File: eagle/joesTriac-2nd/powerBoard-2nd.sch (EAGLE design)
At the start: 31 parts, among them IC1 7809, IC2 7805, IC3 7909, IC5 7805, J1 XF2E-0815-1, J2 XF2E-0815-1

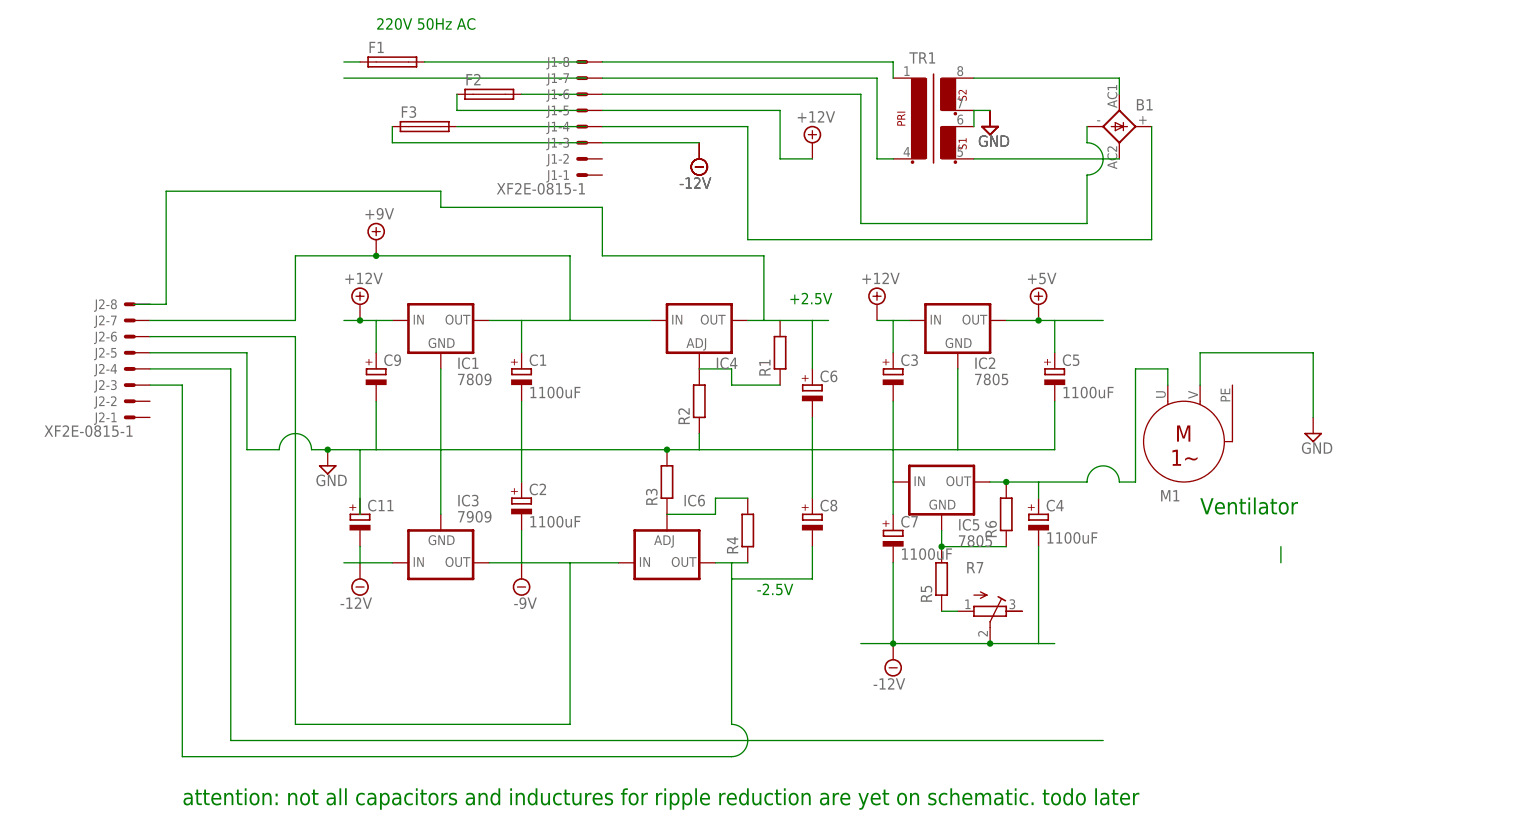
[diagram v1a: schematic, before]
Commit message: reg save-tested ok
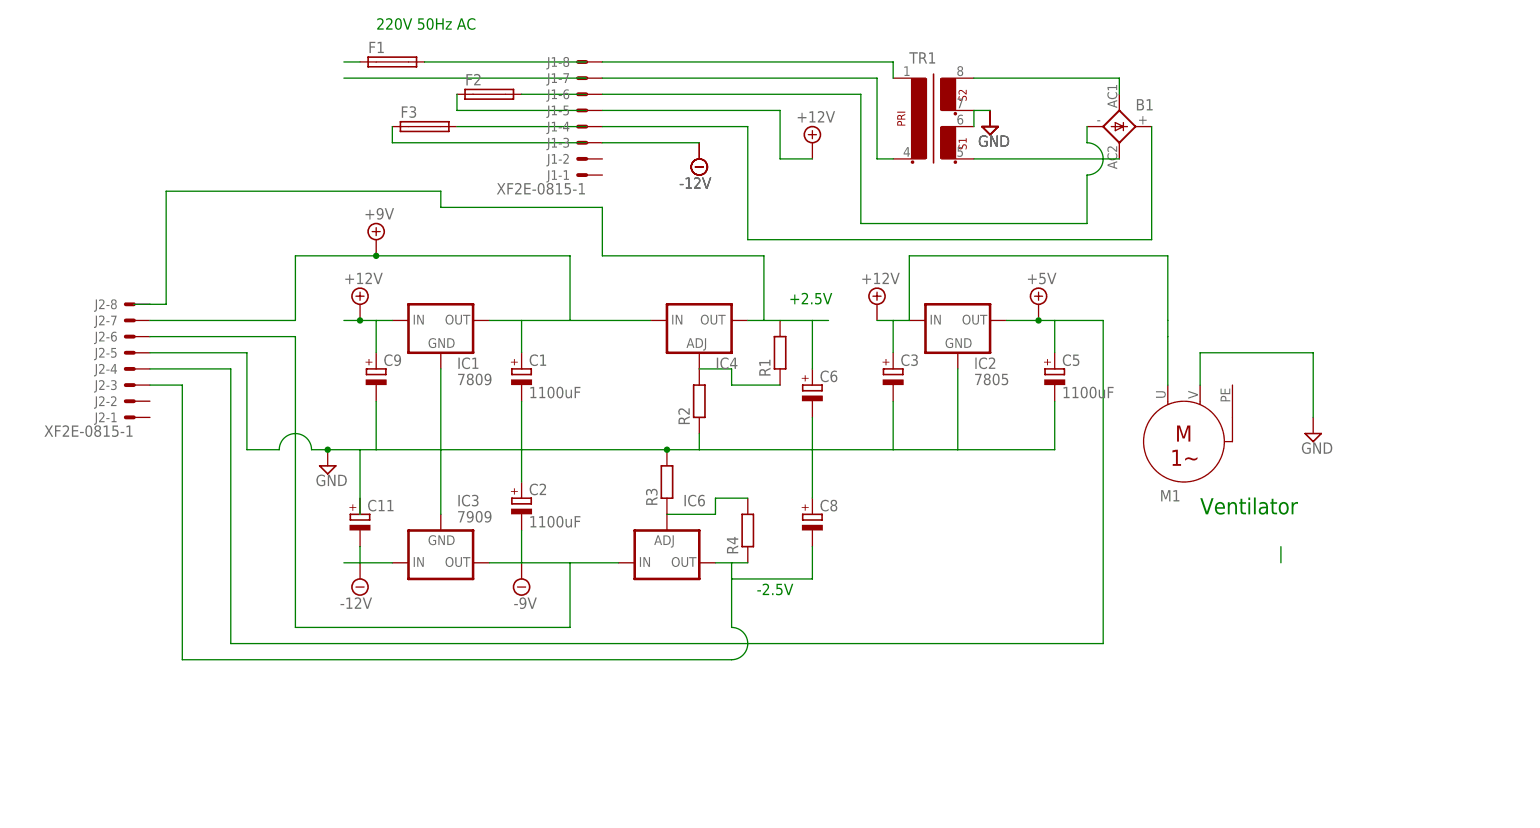
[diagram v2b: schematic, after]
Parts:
- removed C4, C7: 1100uF, resistor:CPOL-EUE22-6AXIAL
- removed IC5: 7805, v-reg:78LXX
- removed R5, R6: (no value), resistor:R-EU_0309/V
- removed R7: (no value), resistor:R-TRIMM3103
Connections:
- removed net N$10: J2-4.MS
- removed net N$16: C4.+, IC5.OUT, M1.U, R6.2
- removed net N$17: R5.1, R7.A
- removed net N$20: IC5.GND, R5.2, R6.1
- net +12V: now also M1.U
- net +5V: now also J2-4.MS
- net -12V: no longer C4.-, C7.-, R7.S
- net GND: no longer C7.+, IC5.IN
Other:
- note removed: "attention: not all capacitors and inductures for ripple reduction are yet on schematic. todo later"
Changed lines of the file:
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@@
 <layer number="97" name="Info" color="7" fill="1" visible="yes" active="yes"/>
 <layer number="98" name="Guide" color="6" fill="1" visible="yes" active="yes"/>
-<layer number="99" name="SpiceOrder" color="5" fill="1" visible="yes" active="yes"/>
 </layers>
 <schematic xreflabel="%F%N/%S.%C%R" xrefpart="/%S.%C%R">
@@
 <part name="SUPPLY13" library="supply2" deviceset="+5V" device=""/>
 <part name="C5" library="resistor" deviceset="CPOL-EU" device="E22-6AXIAL" value="1100uF"/>
-<part name="IC5" library="v-reg" deviceset="78LXX" device="" value="7805"/>
-<part name="SUPPLY14" library="supply2" deviceset="-12V" device=""/>
-<part name="C4" library="resistor" deviceset="CPOL-EU" device="E22-6AXIAL" value="1100uF"/>
-<part name="C7" library="resistor" deviceset="CPOL-EU" device="E22-6AXIAL" value="1100uF"/>
-<part name="R5" library="resistor" deviceset="R-EU_" device="0309/V"/>
-<part name="R7" library="resistor" deviceset="R-TRIMM" device="3103"/>
-<part name="R6" library="resistor" deviceset="R-EU_" device="0309/V"/>
 </parts>
 <sheets>
@@
 <text x="76.2" y="-38.1" size="2.54" layer="91">Ventilator</text>
 <text x="5.08" y="-50.8" size="1.778" layer="91">  -2.5V</text>
-<text x="-83.82" y="-83.82" size="2.54" layer="91">attention: not all capacitors and inductures for ripple reduction are yet on schematic. todo later</text>
 </plain>
 <instances>
@@
 <instance part="SUPPLY13" gate="+5V" x="50.8" y="-5.08"/>
 <instance part="C5" gate="G$1" x="53.34" y="-15.24"/>
-<instance part="IC5" gate="1" x="35.56" y="-33.02"/>
-<instance part="SUPPLY14" gate="G$1" x="27.94" y="-60.96"/>
-<instance part="C4" gate="G$1" x="50.8" y="-38.1"/>
-<instance part="C7" gate="G$1" x="27.94" y="-40.64"/>
-<instance part="R5" gate="G$1" x="35.56" y="-48.26" rot="R90"/>
-<instance part="R7" gate="G$1" x="43.18" y="-53.34" rot="R270"/>
-<instance part="R6" gate="G$1" x="45.72" y="-38.1" rot="R90"/>
 </instances>
 <busses>
@@
 <pinref part="C5" gate="G$1" pin="-"/>
 <wire x1="53.34" y1="-27.94" x2="53.34" y2="-20.32" width="0.1524" layer="91"/>
-<wire x1="27.94" y1="-27.94" x2="27.94" y2="-33.02" width="0.1524" layer="91"/>
-<pinref part="IC5" gate="1" pin="IN"/>
-<pinref part="C7" gate="G$1" pin="+"/>
-<wire x1="27.94" y1="-33.02" x2="27.94" y2="-38.1" width="0.1524" layer="91"/>
 </segment>
 </net>
@@
 </segment>
 <segment>
-<pinref part="SUPPLY9" gate="+12V" pin="+12V"/>
 <pinref part="IC2" gate="1" pin="IN"/>
 <wire x1="30.48" y1="-7.62" x2="27.94" y2="-7.62" width="0.1524" layer="91"/>
+<pinref part="SUPPLY9" gate="+12V" pin="+12V"/>
+<pinref part="C3" gate="G$1" pin="+"/>
 <wire x1="27.94" y1="-7.62" x2="25.4" y2="-7.62" width="0.1524" layer="91"/>
-<pinref part="C3" gate="G$1" pin="+"/>
 <wire x1="27.94" y1="-12.7" x2="27.94" y2="-7.62" width="0.1524" layer="91"/>
+<wire x1="30.48" y1="-7.62" x2="30.48" y2="2.54" width="0.1524" layer="91"/>
+<wire x1="30.48" y1="2.54" x2="71.12" y2="2.54" width="0.1524" layer="91"/>
+<pinref part="M1" gate="1" pin="U"/>
+<wire x1="71.12" y1="-7.62" x2="71.12" y2="-10.16" width="0.1524" layer="91"/>
+<wire x1="71.12" y1="-10.16" x2="71.12" y2="-17.78" width="0.1524" layer="91"/>
+<wire x1="71.12" y1="2.54" x2="71.12" y2="-7.62" width="0.1524" layer="91"/>
 </segment>
 </net>
@@
 <pinref part="C11" gate="G$1" pin="-"/>
 <wire x1="-55.88" y1="-43.18" x2="-55.88" y2="-45.72" width="0.1524" layer="91"/>
-</segment>
-<segment>
-<wire x1="22.86" y1="-58.42" x2="27.94" y2="-58.42" width="0.1524" layer="91"/>
-<pinref part="SUPPLY14" gate="G$1" pin="-12V"/>
-<junction x="27.94" y="-58.42"/>
-<pinref part="C7" gate="G$1" pin="-"/>
-<wire x1="27.94" y1="-45.72" x2="27.94" y2="-58.42" width="0.1524" layer="91"/>
-<wire x1="50.8" y1="-58.42" x2="53.34" y2="-58.42" width="0.1524" layer="91"/>
-<pinref part="C4" gate="G$1" pin="-"/>
-<wire x1="50.8" y1="-43.18" x2="50.8" y2="-58.42" width="0.1524" layer="91"/>
-<wire x1="27.94" y1="-58.42" x2="43.18" y2="-58.42" width="0.1524" layer="91"/>
-<pinref part="R7" gate="G$1" pin="S"/>
-<wire x1="43.18" y1="-58.42" x2="50.8" y2="-58.42" width="0.1524" layer="91"/>
-<junction x="43.18" y="-58.42"/>
 </segment>
 </net>
@@
 <wire x1="-35.56" y1="-45.72" x2="-30.48" y2="-45.72" width="0.1524" layer="91"/>
 <wire x1="-22.86" y1="-45.72" x2="-30.48" y2="-45.72" width="0.1524" layer="91"/>
-<wire x1="-22.86" y1="-45.72" x2="-22.86" y2="-71.12" width="0.1524" layer="91"/>
-<wire x1="-22.86" y1="-71.12" x2="-66.04" y2="-71.12" width="0.1524" layer="91"/>
-<wire x1="-66.04" y1="-71.12" x2="-66.04" y2="-10.16" width="0.1524" layer="91"/>
+<wire x1="-22.86" y1="-45.72" x2="-22.86" y2="-55.88" width="0.1524" layer="91"/>
+<wire x1="-22.86" y1="-55.88" x2="-66.04" y2="-55.88" width="0.1524" layer="91"/>
+<wire x1="-66.04" y1="-55.88" x2="-66.04" y2="-10.16" width="0.1524" layer="91"/>
 <pinref part="IC6" gate="1" pin="IN"/>
 <wire x1="-22.86" y1="-45.72" x2="-15.24" y2="-45.72" width="0.1524" layer="91"/>
@@
 <wire x1="0" y1="-45.72" x2="2.54" y2="-45.72" width="0.1524" layer="91"/>
 <wire x1="2.54" y1="-45.72" x2="2.54" y2="-48.26" width="0.1524" layer="91"/>
-<wire x1="2.54" y1="-48.26" x2="2.54" y2="-71.12" width="0.1524" layer="91"/>
-<wire x1="2.54" y1="-71.12" x2="2.54" y2="-76.2" width="0.1524" layer="91" curve="-180"/>
-<wire x1="2.54" y1="-76.2" x2="-83.82" y2="-76.2" width="0.1524" layer="91"/>
-<wire x1="-83.82" y1="-76.2" x2="-83.82" y2="-17.78" width="0.1524" layer="91"/>
+<wire x1="2.54" y1="-48.26" x2="2.54" y2="-55.88" width="0.1524" layer="91"/>
+<wire x1="2.54" y1="-55.88" x2="2.54" y2="-60.96" width="0.1524" layer="91" curve="-180"/>
+<wire x1="2.54" y1="-60.96" x2="-83.82" y2="-60.96" width="0.1524" layer="91"/>
+<wire x1="-83.82" y1="-60.96" x2="-83.82" y2="-17.78" width="0.1524" layer="91"/>
 <pinref part="J2" gate="-3" pin="MS"/>
 <wire x1="-83.82" y1="-17.78" x2="-88.9" y2="-17.78" width="0.1524" layer="91"/>
@@
 <net name="+5V" class="0">
 <segment>
+<pinref part="IC2" gate="1" pin="OUT"/>
+<wire x1="45.72" y1="-7.62" x2="50.8" y2="-7.62" width="0.1524" layer="91"/>
+<wire x1="50.8" y1="-7.62" x2="53.34" y2="-7.62" width="0.1524" layer="91"/>
 <wire x1="53.34" y1="-7.62" x2="60.96" y2="-7.62" width="0.1524" layer="91"/>
+<wire x1="60.96" y1="-7.62" x2="60.96" y2="-58.42" width="0.1524" layer="91"/>
+<wire x1="60.96" y1="-58.42" x2="-76.2" y2="-58.42" width="0.1524" layer="91"/>
+<wire x1="-76.2" y1="-58.42" x2="-76.2" y2="-15.24" width="0.1524" layer="91"/>
+<pinref part="J2" gate="-4" pin="MS"/>
+<wire x1="-76.2" y1="-15.24" x2="-88.9" y2="-15.24" width="0.1524" layer="91"/>
+<pinref part="SUPPLY13" gate="+5V" pin="+5V"/>
+<junction x="50.8" y="-7.62"/>
 <pinref part="C5" gate="G$1" pin="+"/>
 <wire x1="53.34" y1="-12.7" x2="53.34" y2="-7.62" width="0.1524" layer="91"/>
-<wire x1="50.8" y1="-7.62" x2="53.34" y2="-7.62" width="0.1524" layer="91"/>
-<pinref part="SUPPLY13" gate="+5V" pin="+5V"/>
-<junction x="50.8" y="-7.62"/>
-<pinref part="IC2" gate="1" pin="OUT"/>
-<wire x1="45.72" y1="-7.62" x2="50.8" y2="-7.62" width="0.1524" layer="91"/>
-</segment>
-</net>
-<net name="N$16" class="0">
-<segment>
-<pinref part="IC5" gate="1" pin="OUT"/>
-<wire x1="45.72" y1="-33.02" x2="50.8" y2="-33.02" width="0.1524" layer="91"/>
-<pinref part="C4" gate="G$1" pin="+"/>
-<wire x1="50.8" y1="-33.02" x2="50.8" y2="-35.56" width="0.1524" layer="91"/>
-<wire x1="50.8" y1="-33.02" x2="58.42" y2="-33.02" width="0.1524" layer="91"/>
-<wire x1="58.42" y1="-33.02" x2="63.5" y2="-33.02" width="0.1524" layer="91" curve="-180"/>
-<wire x1="63.5" y1="-33.02" x2="66.04" y2="-33.02" width="0.1524" layer="91"/>
-<wire x1="66.04" y1="-33.02" x2="66.04" y2="-15.24" width="0.1524" layer="91"/>
-<pinref part="M1" gate="1" pin="U"/>
-<wire x1="71.12" y1="-15.24" x2="71.12" y2="-17.78" width="0.1524" layer="91"/>
-<wire x1="66.04" y1="-15.24" x2="71.12" y2="-15.24" width="0.1524" layer="91"/>
-<pinref part="R6" gate="G$1" pin="2"/>
-<junction x="45.72" y="-33.02"/>
-<wire x1="45.72" y1="-33.02" x2="43.18" y2="-33.02" width="0.1524" layer="91"/>
-</segment>
-</net>
-<net name="N$17" class="0">
-<segment>
-<pinref part="R5" gate="G$1" pin="1"/>
-<pinref part="R7" gate="G$1" pin="A"/>
-<wire x1="35.56" y1="-53.34" x2="38.1" y2="-53.34" width="0.1524" layer="91"/>
-</segment>
-</net>
-<net name="N$20" class="0">
-<segment>
-<pinref part="R6" gate="G$1" pin="1"/>
-<wire x1="45.72" y1="-43.18" x2="35.56" y2="-43.18" width="0.1524" layer="91"/>
-<pinref part="IC5" gate="1" pin="GND"/>
-<pinref part="R5" gate="G$1" pin="2"/>
-<wire x1="35.56" y1="-43.18" x2="35.56" y2="-40.64" width="0.1524" layer="91"/>
-<junction x="35.56" y="-43.18"/>
-</segment>
-</net>
-<net name="N$10" class="0">
-<segment>
-<wire x1="60.96" y1="-73.66" x2="-76.2" y2="-73.66" width="0.1524" layer="91"/>
-<wire x1="-76.2" y1="-73.66" x2="-76.2" y2="-15.24" width="0.1524" layer="91"/>
-<pinref part="J2" gate="-4" pin="MS"/>
-<wire x1="-76.2" y1="-15.24" x2="-88.9" y2="-15.24" width="0.1524" layer="91"/>
-</segment>
-</net>
+</segment>
+</net>
